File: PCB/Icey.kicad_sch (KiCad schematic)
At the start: 113 parts, among them J1 Conn_01x12, J2 Conn_01x08, SW2 TS-1088-AR02016, SW3 TS-1088-AR02016, U1 AMS1117-1.2, U2 ICE40UP5K-SG48I, U3 MAX3421EETJ+T, U4 W25Q128JVSIQTR, U5 AMS1117-3.3, U6 FT2232HL, X1 X322512MSB4SI, X2 X322512MSB4SI

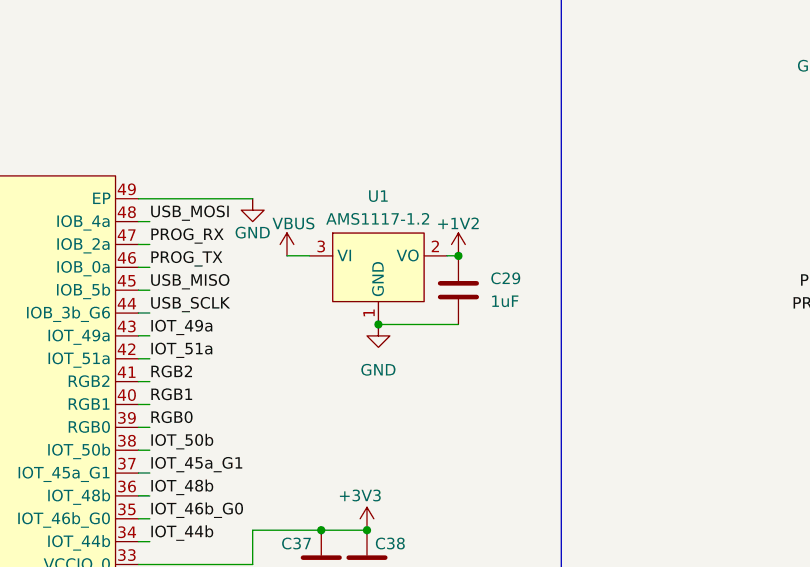
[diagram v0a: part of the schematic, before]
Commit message: done!!
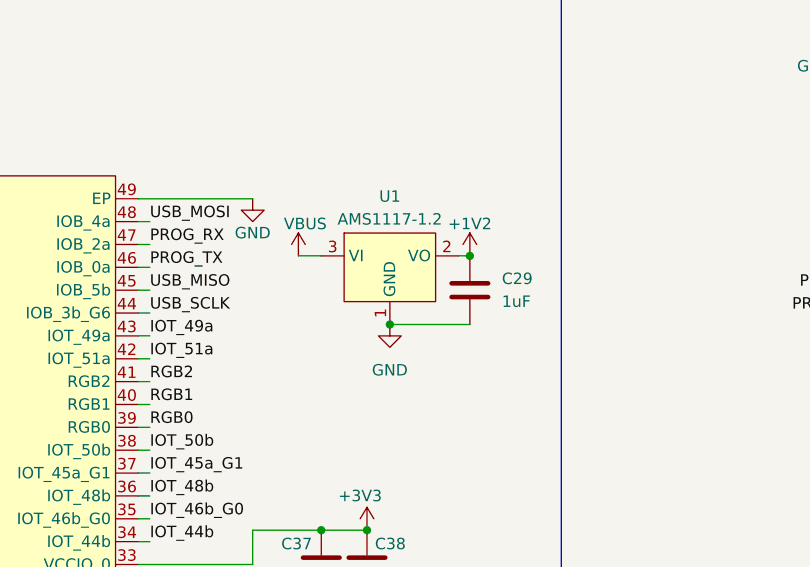
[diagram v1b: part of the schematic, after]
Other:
- moved on the sheet: C29, U1
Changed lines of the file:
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@@
 	)
 	(junction
-		(at 257.81 121.92)
+		(at 259.08 121.92)
 		(diameter 0)
 		(color 0 0 0 0)
@@
 	)
 	(junction
-		(at 266.7 114.3)
+		(at 267.97 114.3)
 		(diameter 0)
 		(color 0 0 0 0)
@@
 	(wire
 		(pts
-			(xy 265.43 114.3) (xy 266.7 114.3)
+			(xy 266.7 114.3) (xy 267.97 114.3)
 		)
 		(stroke
@@
 	(wire
 		(pts
-			(xy 257.81 121.92) (xy 266.7 121.92)
+			(xy 259.08 121.92) (xy 267.97 121.92)
 		)
 		(stroke
@@
 	(wire
 		(pts
-			(xy 247.65 114.3) (xy 250.19 114.3)
+			(xy 248.92 114.3) (xy 251.46 114.3)
 		)
 		(stroke
@@
 	(symbol
 		(lib_id "power:VBUS")
-		(at 247.65 114.3 0)
+		(at 248.92 114.3 0)
 		(unit 1)
 		(exclude_from_sim no)
@@
 		(dnp no)
 		(property "Reference" "#PWR066"
-			(at 247.65 118.11 0)
+			(at 248.92 118.11 0)
 			(effects
 				(font
@@
 		)
 		(property "Value" "VBUS"
-			(at 248.412 110.744 0)
+			(at 249.682 110.744 0)
 			(effects
 				(font
@@
 		)
 		(property "Footprint" ""
-			(at 247.65 114.3 0)
+			(at 248.92 114.3 0)
 			(effects
 				(font
@@
 		)
 		(property "Datasheet" ""
-			(at 247.65 114.3 0)
+			(at 248.92 114.3 0)
 			(effects
 				(font
@@
 		)
 		(property "Description" "Power symbol creates a global label with name \"VBUS\""
-			(at 247.65 114.3 0)
+			(at 248.92 114.3 0)
 			(effects
 				(font
@@
 	(symbol
 		(lib_id "power:+1V2")
-		(at 266.7 114.3 0)
+		(at 267.97 114.3 0)
 		(unit 1)
 		(exclude_from_sim no)
@@
 		(dnp no)
 		(property "Reference" "#PWR012"
-			(at 266.7 118.11 0)
+			(at 267.97 118.11 0)
 			(effects
 				(font
@@
 		)
 		(property "Value" "+1V2"
-			(at 266.7 110.744 0)
+			(at 267.97 110.744 0)
 			(effects
 				(font
@@
 		)
 		(property "Footprint" ""
-			(at 266.7 114.3 0)
+			(at 267.97 114.3 0)
 			(effects
 				(font
@@
 		)
 		(property "Datasheet" ""
-			(at 266.7 114.3 0)
+			(at 267.97 114.3 0)
 			(effects
 				(font
@@
 		)
 		(property "Description" "Power symbol creates a global label with name \"+1V2\""
-			(at 266.7 114.3 0)
+			(at 267.97 114.3 0)
 			(effects
 				(font
@@
 	(symbol
 		(lib_id "power:GND")
-		(at 257.81 121.92 0)
+		(at 259.08 121.92 0)
 		(unit 1)
 		(exclude_from_sim no)
@@
 		(fields_autoplaced yes)
 		(property "Reference" "#PWR027"
-			(at 257.81 128.27 0)
+			(at 259.08 128.27 0)
 			(effects
 				(font
@@
 		)
 		(property "Value" "GND"
-			(at 257.81 127 0)
+			(at 259.08 127 0)
 			(effects
 				(font
@@
 		)
 		(property "Footprint" ""
-			(at 257.81 121.92 0)
+			(at 259.08 121.92 0)
 			(effects
 				(font
@@
 		)
 		(property "Datasheet" ""
-			(at 257.81 121.92 0)
+			(at 259.08 121.92 0)
 			(effects
 				(font
@@
 		)
 		(property "Description" "Power symbol creates a global label with name \"GND\" , ground"
-			(at 257.81 121.92 0)
+			(at 259.08 121.92 0)
 			(effects
 				(font
@@
 	(symbol
 		(lib_id "Device:C")
-		(at 266.7 118.11 0)
+		(at 267.97 118.11 0)
 		(unit 1)
 		(exclude_from_sim no)
@@
 		(dnp no)
 		(property "Reference" "C29"
-			(at 270.256 116.84 0)
+			(at 271.526 116.84 0)
 			(effects
 				(font
@@
 		)
 		(property "Value" "1uF"
-			(at 270.256 119.38 0)
+			(at 271.526 119.38 0)
 			(effects
 				(font
@@
 		)
 		(property "Footprint" "Capacitor_SMD:C_0603_1608Metric"
-			(at 267.6652 121.92 0)
+			(at 268.9352 121.92 0)
 			(effects
 				(font
@@
 		)
 		(property "Datasheet" "~"
-			(at 266.7 118.11 0)
+			(at 267.97 118.11 0)
 			(effects
 				(font
@@
 		)
 		(property "Description" "Unpolarized capacitor"
-			(at 266.7 118.11 0)
+			(at 267.97 118.11 0)
 			(effects
 				(font
@@
 	(symbol
 		(lib_id "easyeda2kicad:AMS1117-1.2_C347218")
-		(at 257.81 115.57 0)
+		(at 259.08 115.57 0)
 		(unit 1)
 		(exclude_from_sim no)
@@
 		(dnp no)
 		(property "Reference" "U1"
-			(at 257.81 107.696 0)
+			(at 259.08 107.696 0)
 			(effects
 				(font
@@
 		)
 		(property "Value" "AMS1117-1.2"
-			(at 257.81 110.236 0)
+			(at 259.08 110.236 0)
 			(effects
 				(font
@@
 		)
 		(property "Footprint" "Package_TO_SOT_SMD:SOT-223-3_TabPin2"
-			(at 257.81 125.73 0)
+			(at 259.08 125.73 0)
 			(effects
 				(font
@@
 		)
 		(property "Datasheet" "https://lcsc.com/product-detail/Others_Youtai-Semiconductor-Co-Ltd-AMS1117-1-2_C347218.html"
-			(at 257.81 128.27 0)
+			(at 259.08 128.27 0)
 			(effects
 				(font
@@
 		)
 		(property "Description" ""
-			(at 257.81 115.57 0)
+			(at 259.08 115.57 0)
 			(effects
 				(font
@@
 		)
 		(property "Manufacturer" "UMW(友台半导体)"
-			(at 257.81 130.81 0)
+			(at 259.08 130.81 0)
 			(effects
 				(font
@@
 		)
 		(property "MPN" "AMS1117-1.2"
-			(at 257.81 133.35 0)
+			(at 259.08 133.35 0)
 			(effects
 				(font
@@
 		)
 		(property "LCSC Part" "C347218"
-			(at 257.81 135.89 0)
+			(at 259.08 135.89 0)
 			(effects
 				(font
